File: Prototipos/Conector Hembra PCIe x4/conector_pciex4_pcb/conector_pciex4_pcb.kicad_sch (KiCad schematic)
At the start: 33 parts, among them J1 10018783-10211TLF

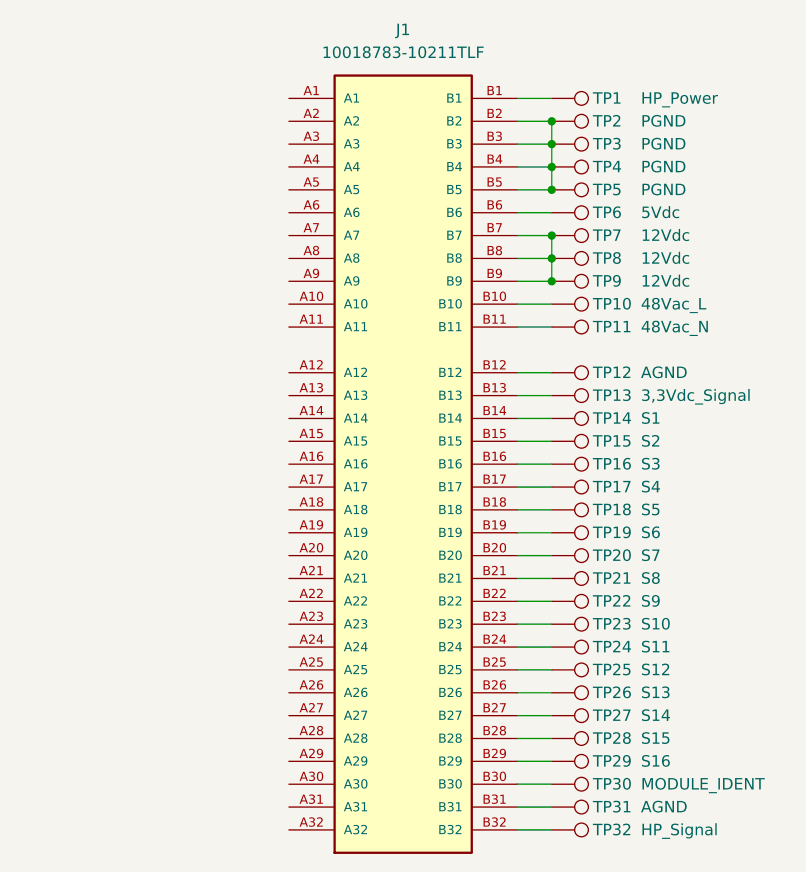
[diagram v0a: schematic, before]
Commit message: Corrección PCB
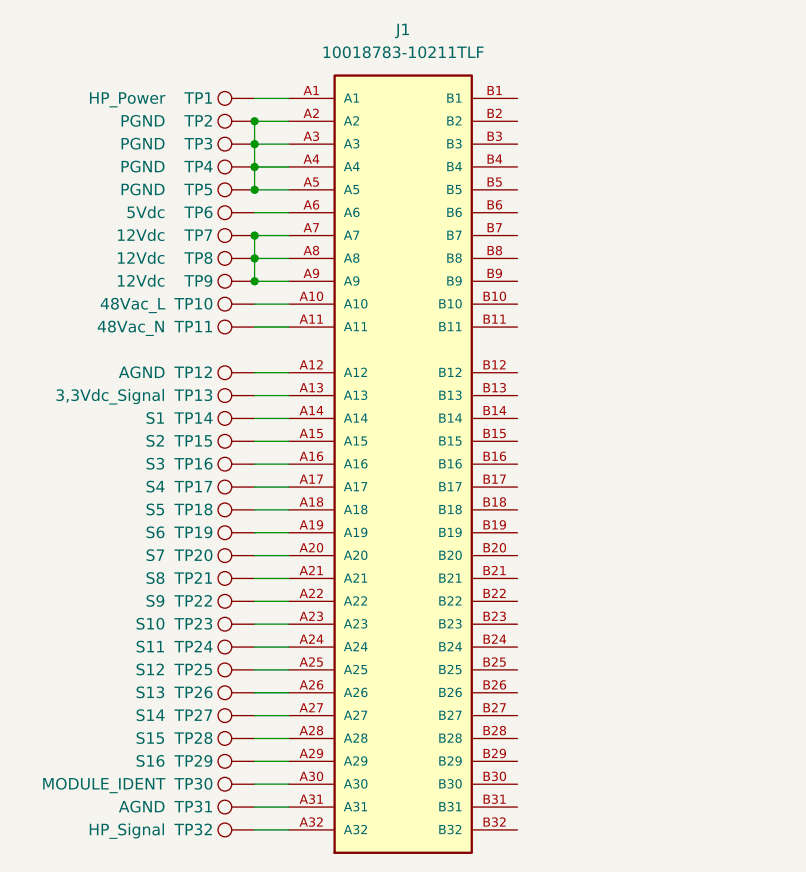
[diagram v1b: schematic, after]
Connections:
- net at TP20.1: now also J1.A20; no longer J1.B20
- net at TP25.1: now also J1.A25; no longer J1.B25
- net at TP32.1: now also J1.A32; no longer J1.B32
- net at TP31.1: now also J1.A31; no longer J1.B31
- net at TP26.1: now also J1.A26; no longer J1.B26
- net at TP13.1: now also J1.A13; no longer J1.B13
- net at TP12.1: now also J1.A12; no longer J1.B12
- net at TP16.1: now also J1.A16; no longer J1.B16
- net at TP29.1: now also J1.A29; no longer J1.B29
- net at TP22.1: now also J1.A22; no longer J1.B22
- net at TP2.1, TP3.1, TP4.1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: now also J1.A2, J1.A3, J1.A4, J1.A5; no longer J1.B2, J1.B3, J1.B4, J1.B5
- net at TP28.1: now also J1.A28; no longer J1.B28
- net at TP1.1: now also J1.A1; no longer J1.B1
- net at TP15.1: now also J1.A15; no longer J1.B15
- net at TP6.1: now also J1.A6; no longer J1.B6
- net at TP17.1: now also J1.A17; no longer J1.B17
- net at TP10.1: now also J1.A10; no longer J1.B10
- net at TP21.1: now also J1.A21; no longer J1.B21
- net at TP19.1: now also J1.A19; no longer J1.B19
- net at TP7.1, TP8.1, TP9.1: now also J1.A7, J1.A8, J1.A9; no longer J1.B7, J1.B8, J1.B9
- net at TP11.1: now also J1.A11; no longer J1.B11
- net at TP18.1: now also J1.A18; no longer J1.B18
- net at J1.A14: now also TP14.1
- net at J1.A23: now also TP23.1
- net at J1.A24: now also TP24.1
- net at J1.A27: now also TP27.1
- net at J1.A30: now also TP30.1
- net at J1.B14: no longer TP14.1
- net at J1.B23: no longer TP23.1
- net at J1.B24: no longer TP24.1
- net at J1.B27: no longer TP27.1
- net at J1.B30: no longer TP30.1
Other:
- moved on the sheet: TP1, TP10, TP11, TP12, TP13, TP14, TP15, TP16, TP17, TP18, TP19, TP2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
